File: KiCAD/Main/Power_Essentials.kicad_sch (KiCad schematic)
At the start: 29 parts, among them J1 USB_C_Receptacle_USB2.0_16P, J2 Micro_SD_Card_Det2, J4 Screw_Terminal_01x09, J5 Screw_Terminal_01x09, Q1 BC108, Q2 BC108, Q3 BC108, SW1 RESET, SW2 USER, U2 LM2596S-3.3, U3 LM2596S-5, U4 TPS2121RUXR

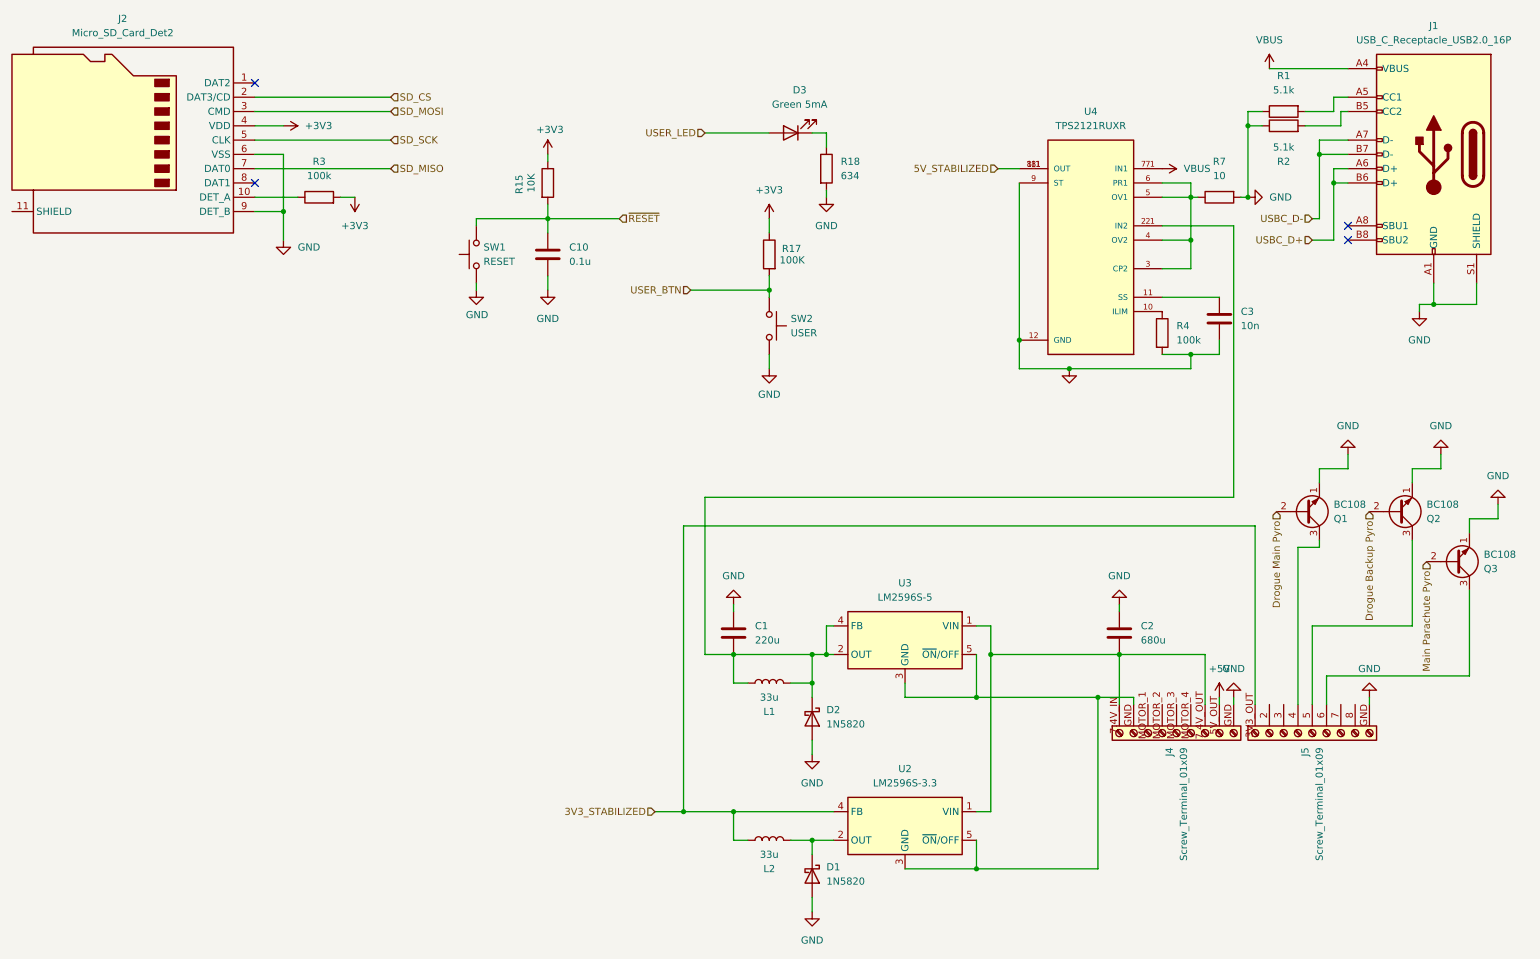
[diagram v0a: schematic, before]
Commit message: Keep up to date
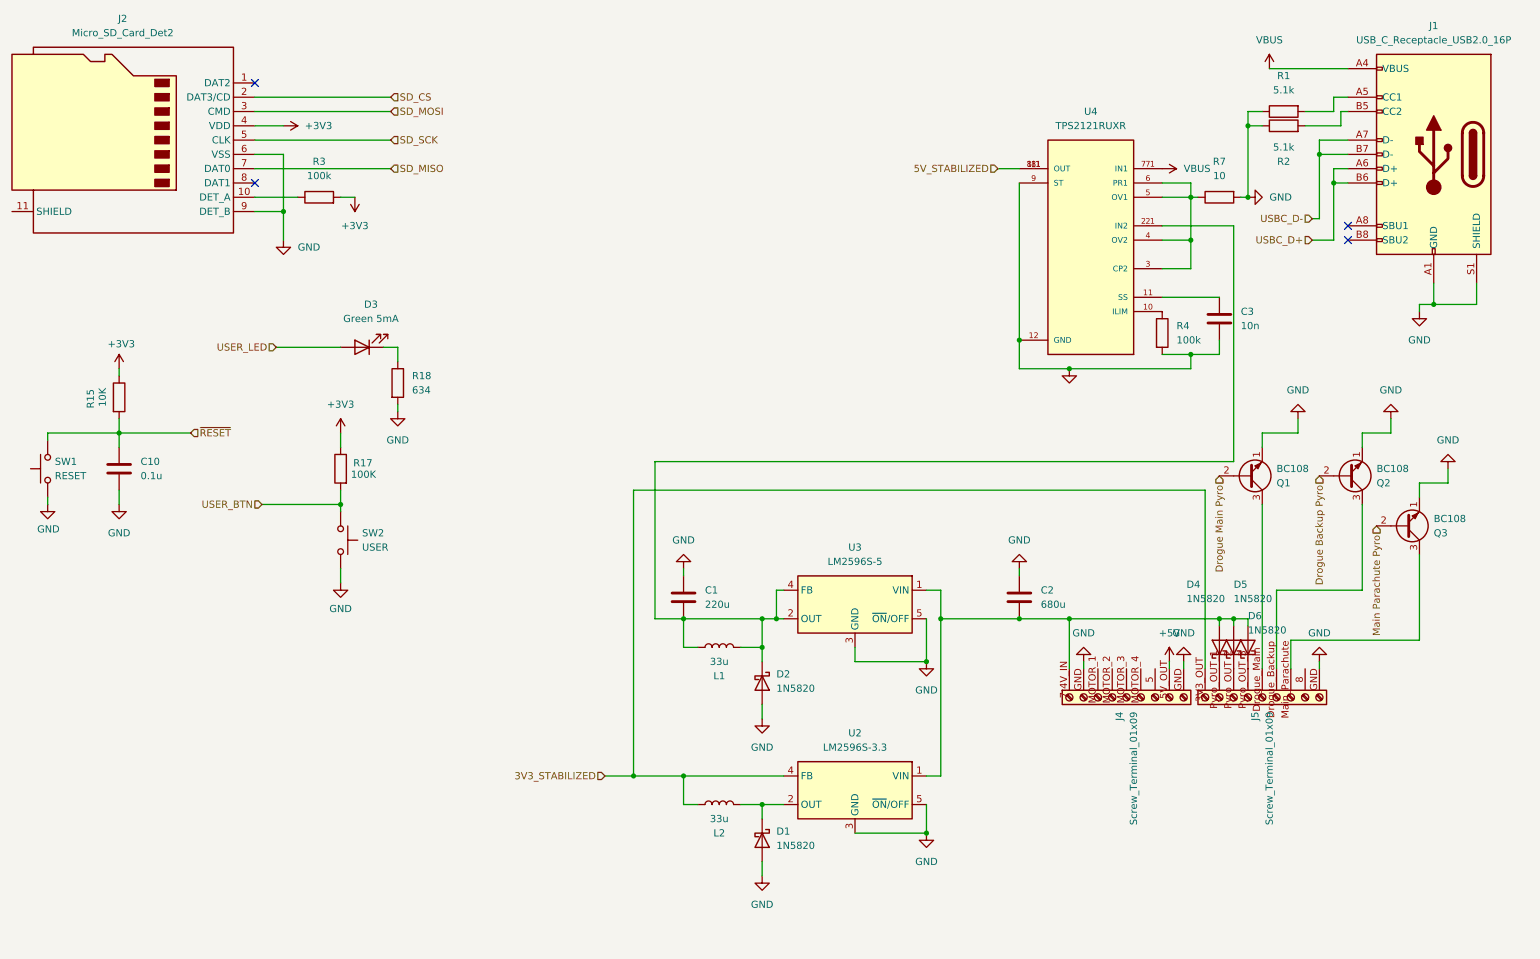
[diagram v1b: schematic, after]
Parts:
- added D4, D5, D6: 1N5820, Diode_THT:D_DO-201AD_P15.24mm_Horizontal, symbol Diode:1N5820
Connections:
- net GND: now also U2.3 (GND), U2.5 (~{ON}/OFF), U3.3 (GND), U3.5 (~{ON}/OFF)
- net at Q3.3 (C): now also J5.Main_Parachute; no longer J5.6 (Pin_6)
- net at C2.2, J4.7.4V_IN, U2.1 (VIN)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: now also D4.2 (A), D5.2 (A), D6.2 (A); no longer J4.7.4V_OUT
- net at Q2.3 (C): now also J5.Drogue_Backup; no longer J5.5 (Pin_5)
- net at Q1.3 (C): now also J5.Drogue_Main; no longer J5.4 (Pin_4)
- new net: D4.1 (K), J5.Pyro_OUT_1
- new net: D6.1 (K), J5.Pyro_OUT_3
- new net: D5.1 (K), J5.Pyro_OUT_2
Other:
- moved on the sheet: C1, C10, C2, D1, D2, D3, J4, J5, L1, L2, Q1, Q2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
